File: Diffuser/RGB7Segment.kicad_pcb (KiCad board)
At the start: 2 copper layers, 35.2 x 11.7 mm, 2 parts, among them J1 Conn_01x02_Socket, J2 Conn_01x04_Pin

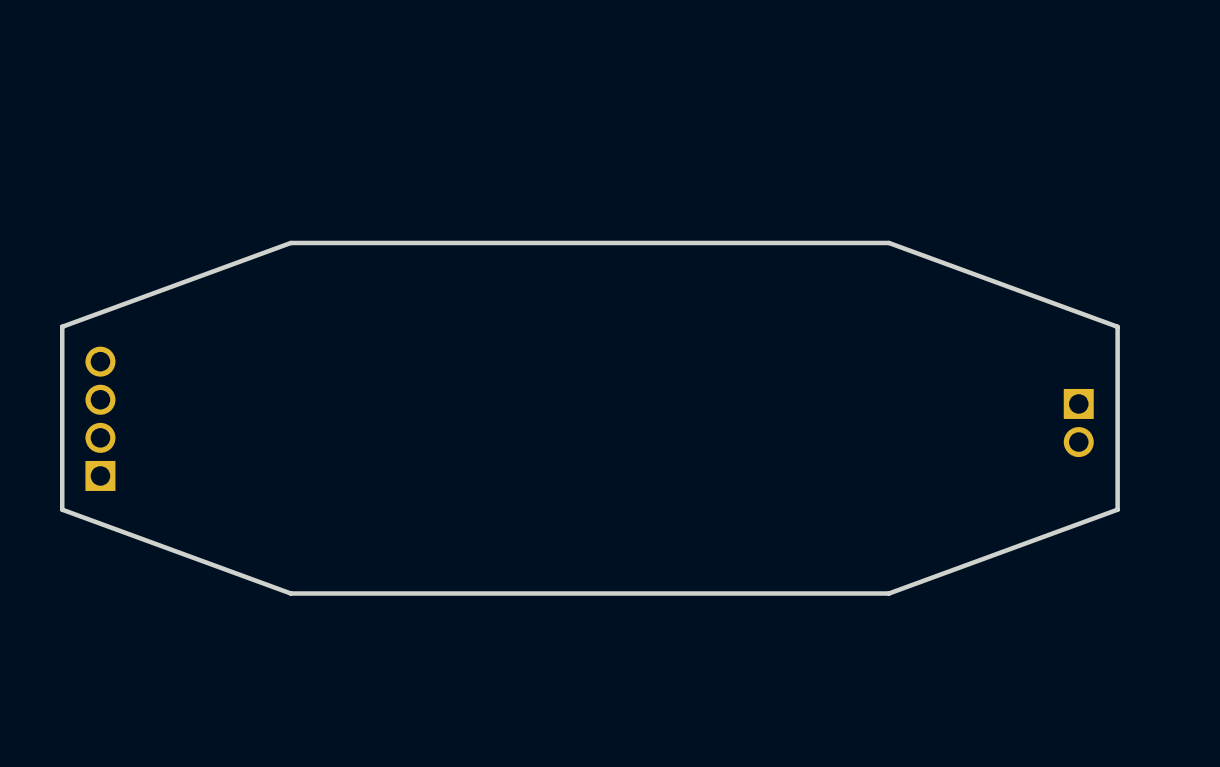
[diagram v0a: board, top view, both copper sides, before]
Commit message: New Layout for diffuser. Needs further direction.
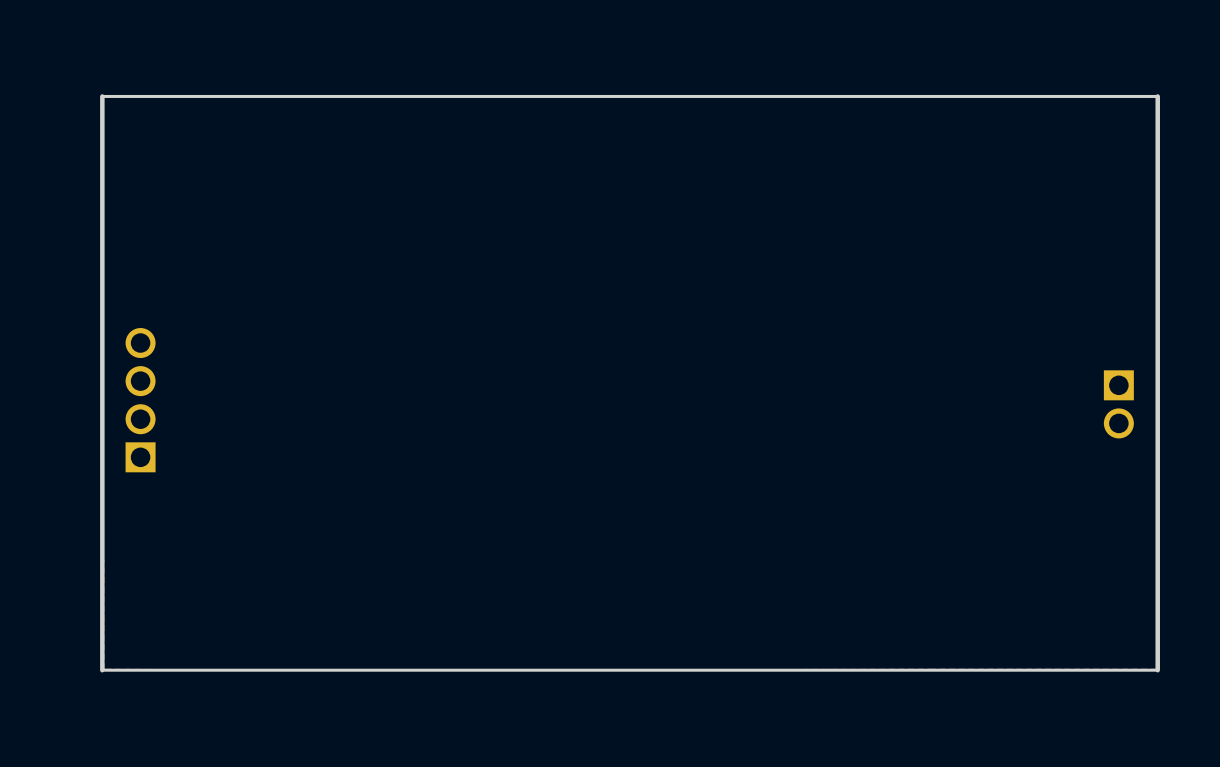
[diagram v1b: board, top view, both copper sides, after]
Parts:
- moved J1 1.47 mm to (252.1, 105.3)
- moved J2 1.47 mm to (219.5, 107.7)
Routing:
- added copper zone on B.Cu, net GND
- added copper zone on F.Cu, net GND
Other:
- board size 35.2 x 11.7 mm -> 35.2 x 19.1 mm
- board text added: "GND"
- board text added: "VCC"

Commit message: New Minor Layout
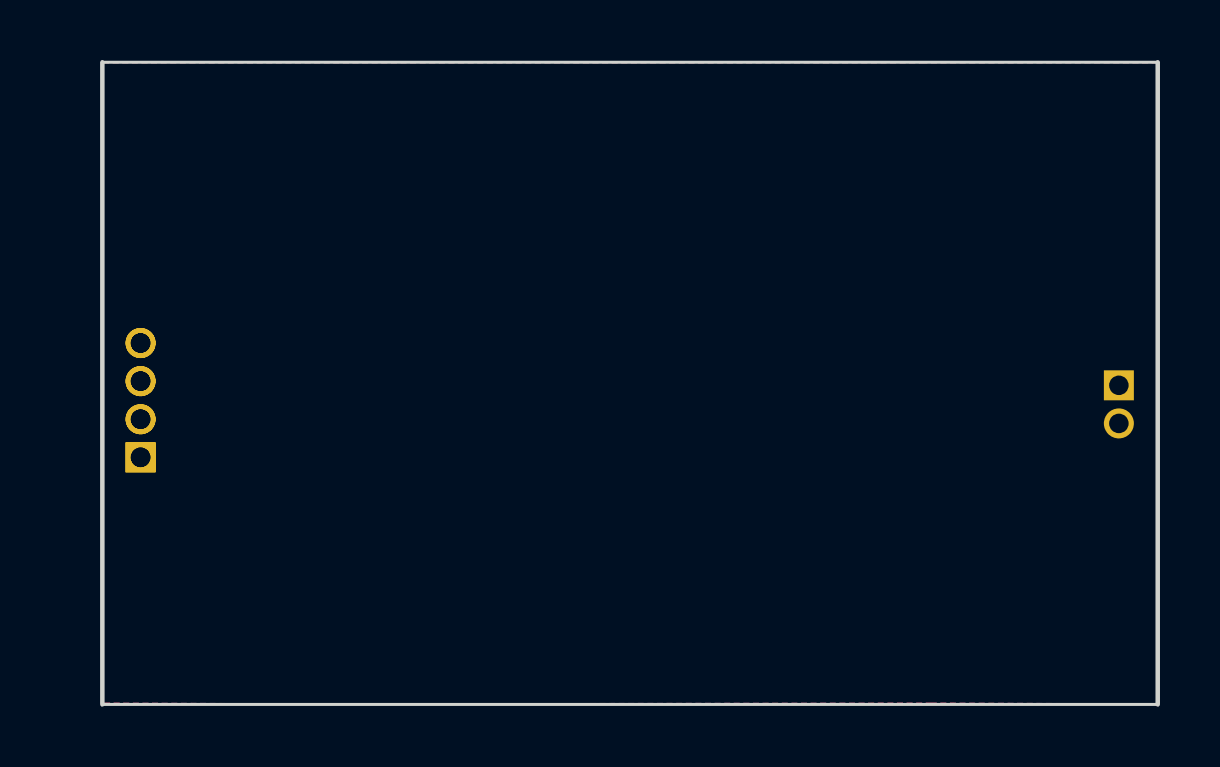
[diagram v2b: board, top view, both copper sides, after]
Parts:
- added J2: Conn_01x04_Pin, Connector_PinHeader_1.27mm:PinHeader_1x04_P1.27mm_Vertical, B.Cu at (219.5, 107.7)
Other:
- board size 35.2 x 19.1 mm -> 35.2 x 21.4 mm
